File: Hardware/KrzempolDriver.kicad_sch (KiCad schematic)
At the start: 42 parts, among them J1 24V, U1 RT6285, U2 RT6285, U3 RT6285

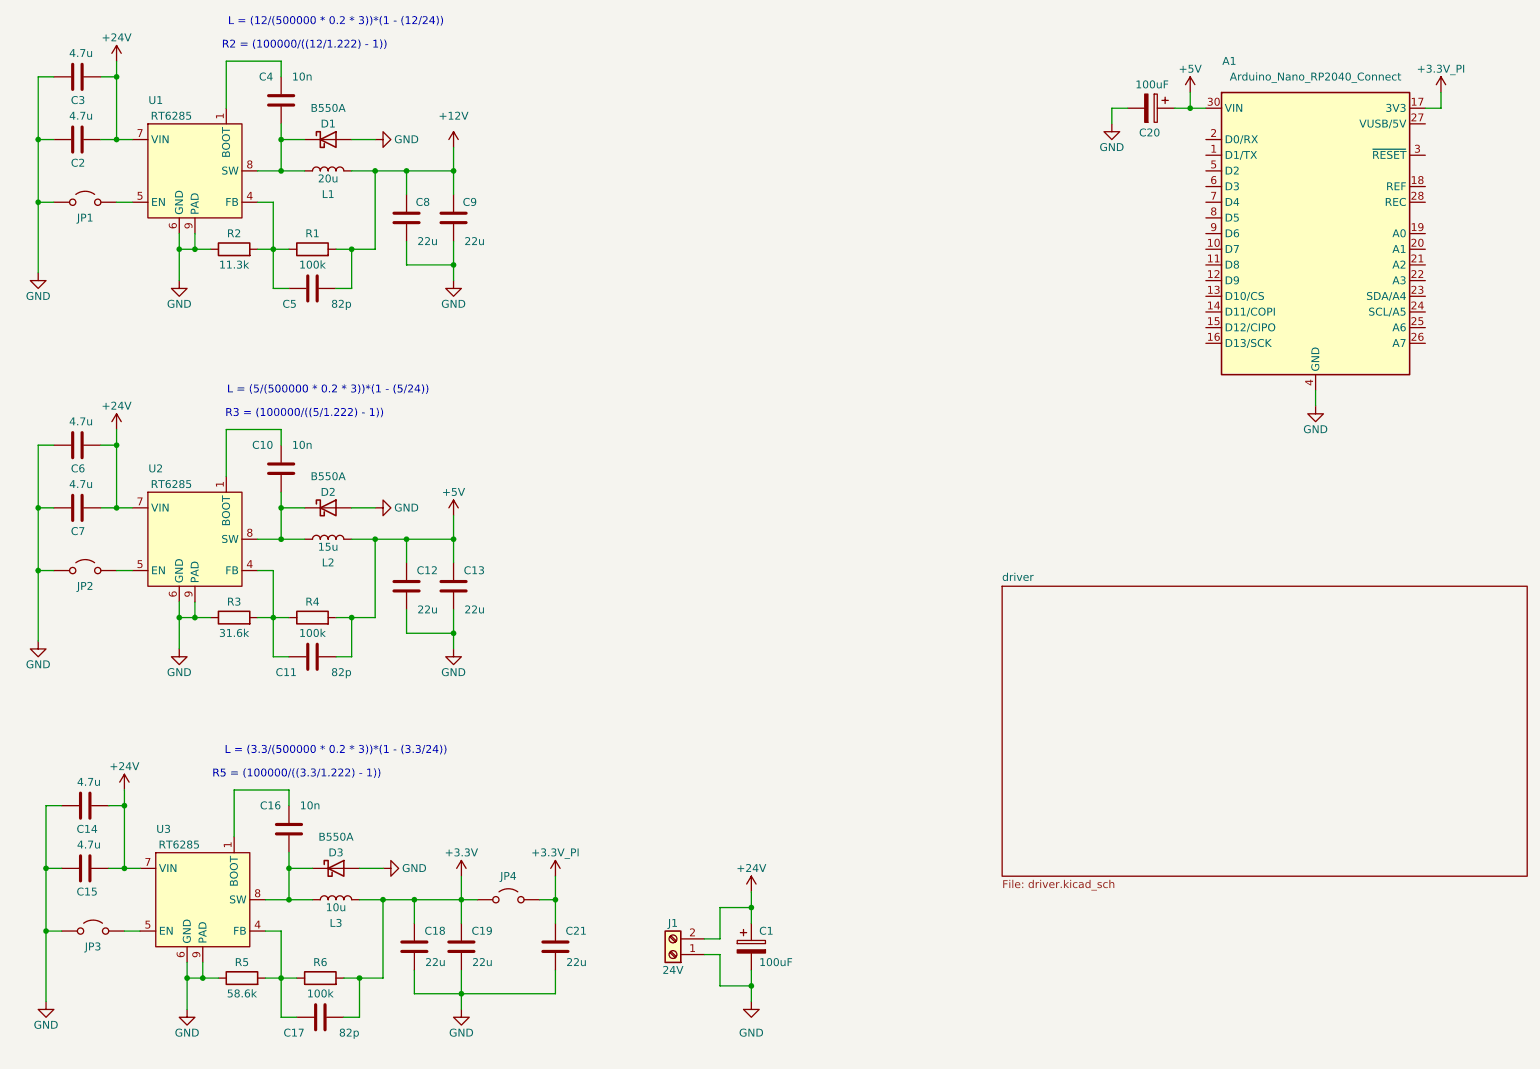
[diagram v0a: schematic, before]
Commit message: driver and output
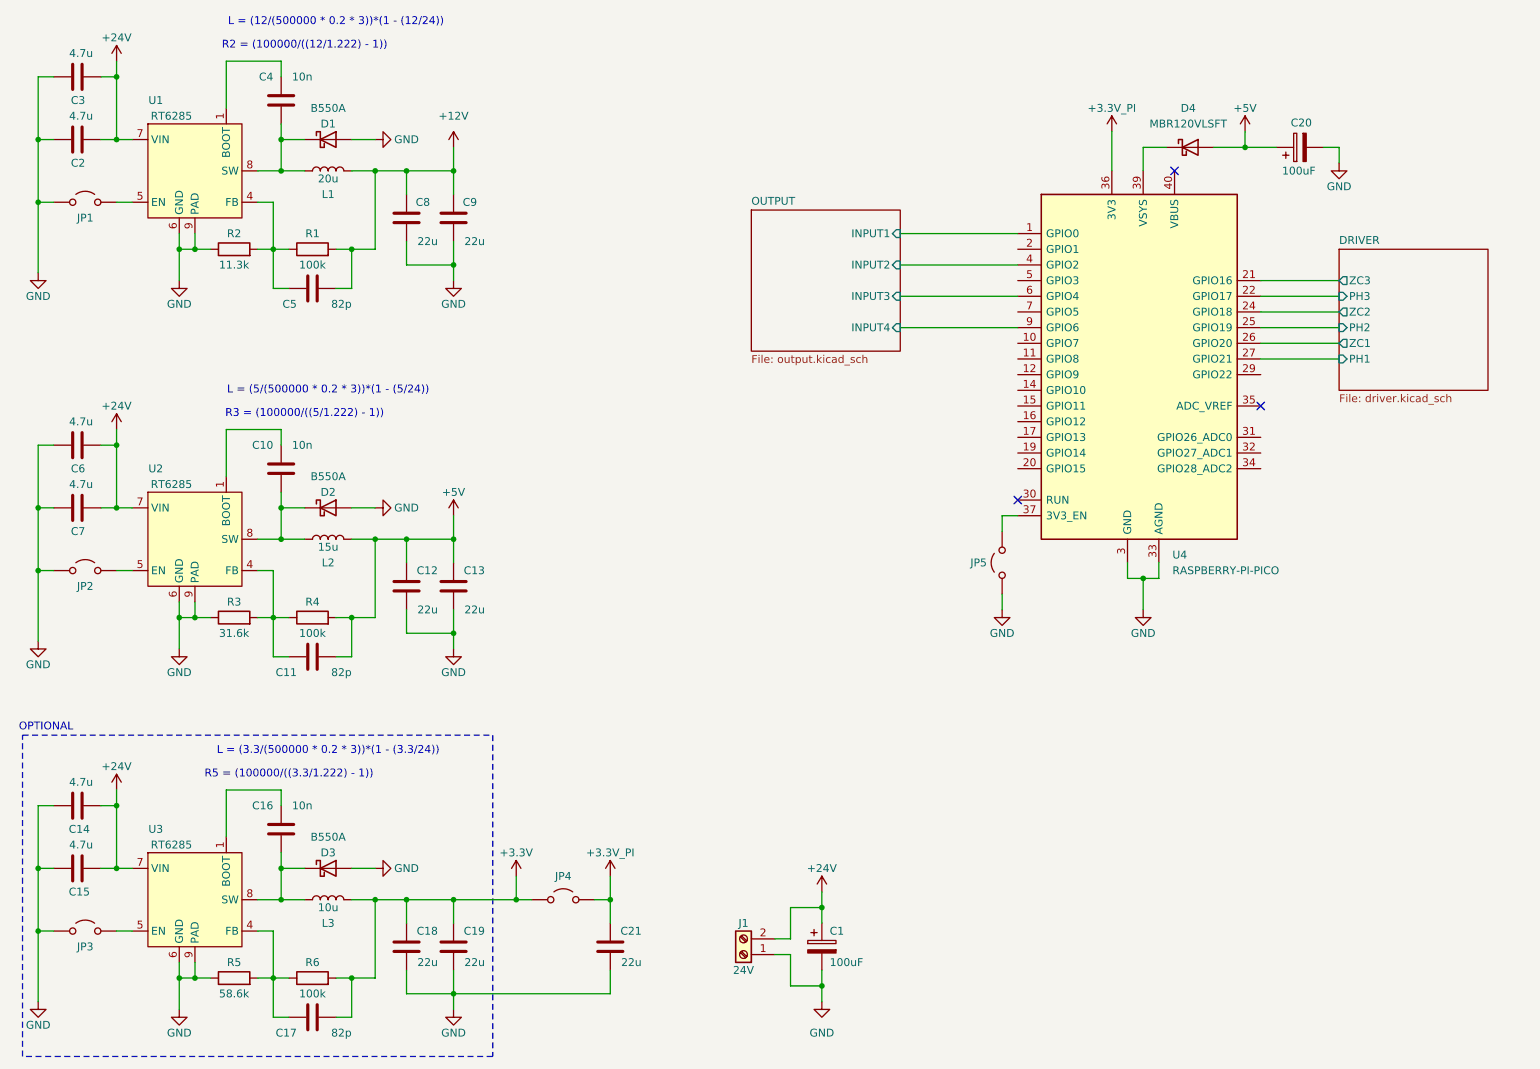
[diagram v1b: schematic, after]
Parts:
- removed A1: Arduino_Nano_RP2040_Connect, Module:Arduino_Nano, symbol MCU_Module:Arduino_Nano_RP2040_Connect
- added D4: MBR120VLSFT, symbol Device:D_Schottky
- added JP5: Jumper_2_Open, symbol Jumper:Jumper_2_Open
- added U4: RASPBERRY-PI-PICO, Module_RaspberryPi_Pico:RaspberryPi_Pico_Common, symbol krzempol:RASPBERRY-PI-PICO
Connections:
- net +3.3V_PI: now also U4.36 (3V3)
- net +5V: now also D4.2 (A)
- net GND: now also JP5.1 (A), U4.13 (GND), U4.18 (GND), U4.23 (GND), U4.28 (GND), U4.3 (GND), U4.33 (AGND), U4.38 (GND), U4.8 (GND)
- new net: JP5.2 (B), U4.37 (3V3_EN)
- new net: D4.1 (K), U4.39 (VSYS)
- new net DRIVER/PH1: U4.27 (GPIO21)
- new net DRIVER/PH2: U4.25 (GPIO19)
- new net DRIVER/PH3: U4.22 (GPIO17)
- new net DRIVER/ZC1: U4.26 (GPIO20)
- new net DRIVER/ZC2: U4.24 (GPIO18)
- new net DRIVER/ZC3: U4.21 (GPIO16)
- new net OUTPUT/INPUT1: U4.1 (GPIO0)
- new net OUTPUT/INPUT2: U4.4 (GPIO2)
- new net OUTPUT/INPUT3: U4.6 (GPIO4)
- new net OUTPUT/INPUT4: U4.9 (GPIO6)
- no-connect marks 0 -> 3
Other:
- sheet driver renamed DRIVER
- added sheet OUTPUT (output.kicad_sch)
- sheet DRIVER ports: added PH1, PH2, PH3, ZC1, ZC2, ZC3; removed none
- note added: "OPTIONAL"
- moved on the sheet: C1, C14, C15, C16, C17, C18, C19, C20, C21, D3, J1, JP3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
